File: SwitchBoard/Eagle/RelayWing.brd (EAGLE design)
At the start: 51.7 x 55.9 mm, 30 parts, among them K1 EE2-3TNUH, K2 EE2-3TNUH, K3 EE2-3TNUH, K4 EE2-3TNUH, K5 EE2-3TNUH, U1 ULN2003ANS, U2 ULN2003ANS, U3 MCP23017SS, U4 INA219AID

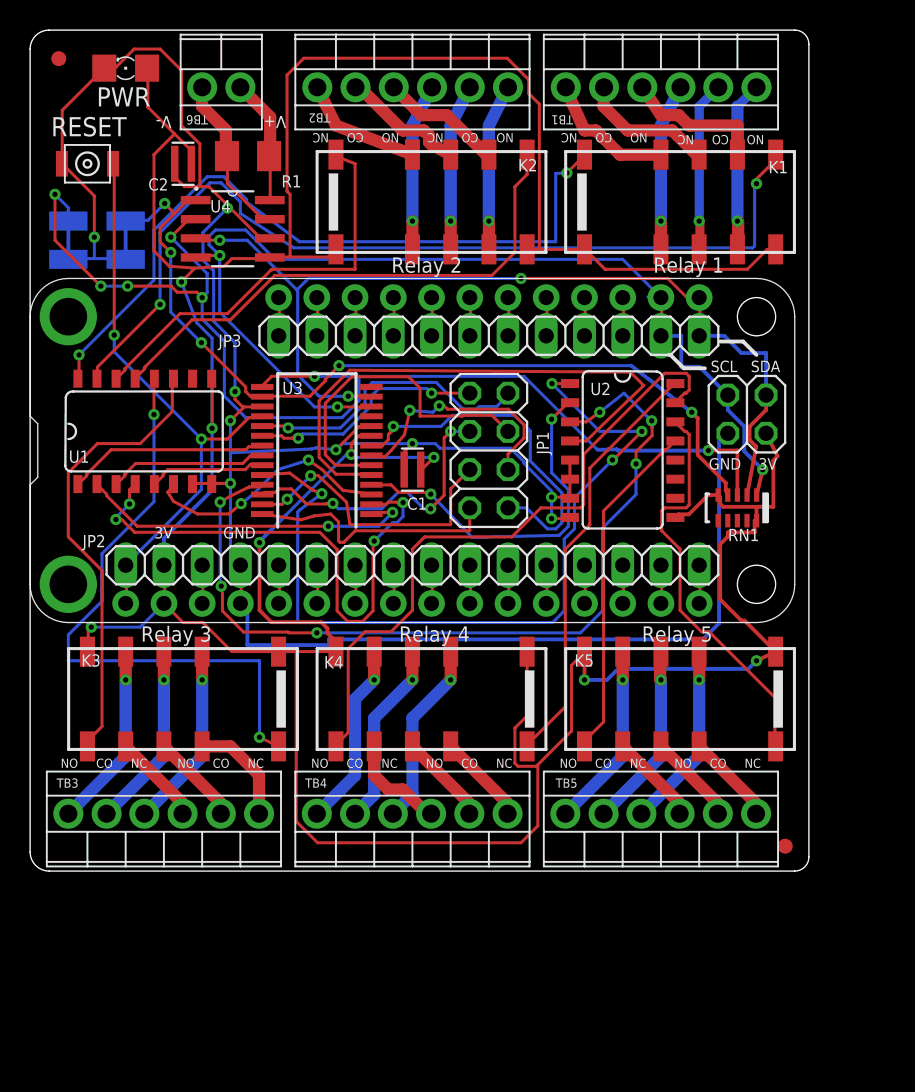
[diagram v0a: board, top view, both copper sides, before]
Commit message: Rev B (start)
First commit for Rev B. See updated Description.
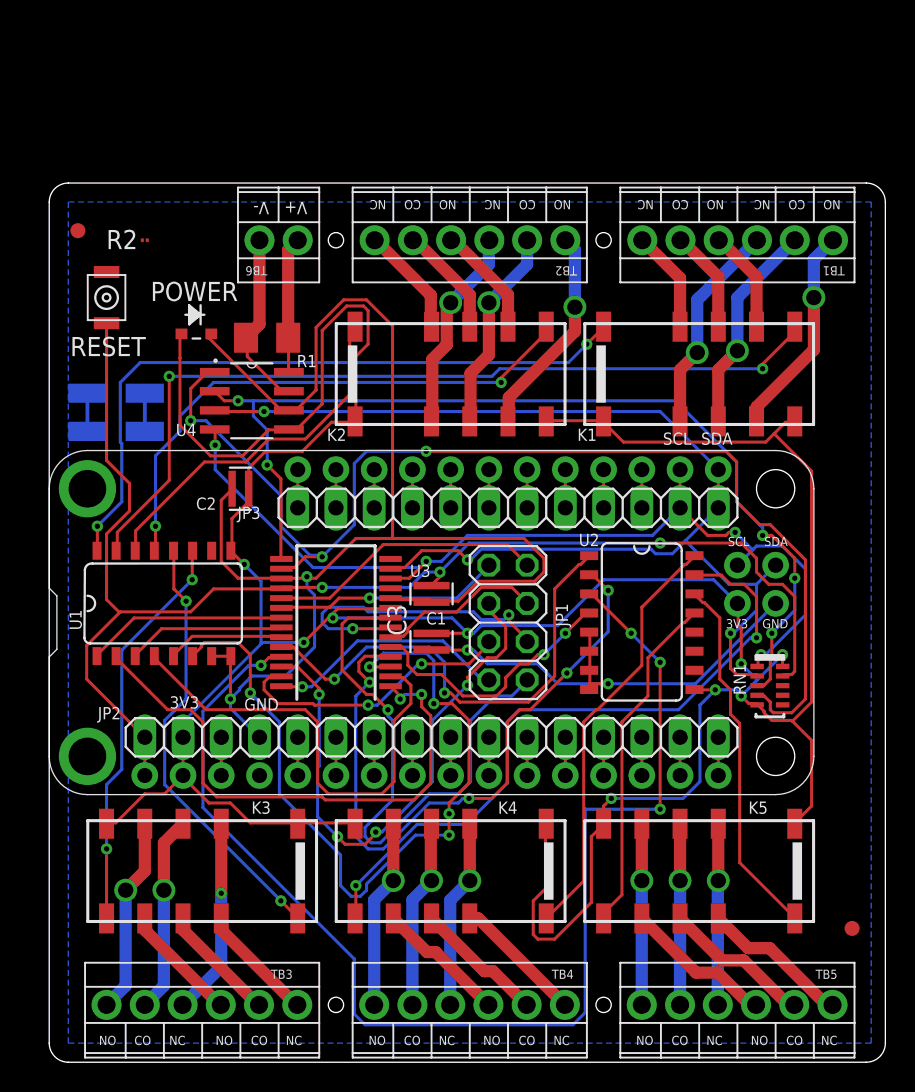
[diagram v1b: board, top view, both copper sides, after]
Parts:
- removed I2CHDR: (no value), pinhead:2X02
- removed PWR: (no value), led:1206
- added C3: MUR-1220-CAP, home:CAPC2012
- added JP4, JP5, JP6, JP7: (no value), adafruit:1X01-CLEANBIG
- added POWER: HSMQ-C191, DigiKey:LED3_HSMX-C120
- added R2: 330, home:R01005
- RN1: value CTS746X101 -> CTS746X101102JP
- moved C2 21.9 mm to (14.0, 39.4)
- moved TB5 13.7 mm to (47.0, 5.08)
- moved TB4 13.3 mm to (29.2, 5.08)
- moved TB3 13.0 mm to (11.4, 5.08)
- moved R1 12.1 mm to (15.7, 49.4)
- moved RN1 12.0 mm to (49.1, 26.3), turned to 270 degrees
- moved A0 11.5 mm to (3.81, 44.5)
- moved A1 11.5 mm to (7.62, 44.5)
- moved C1 11.5 mm to (26.7, 29.2), turned to 270 degrees
- moved JP2 11.5 mm to (26.7, 22.9)
- moved JP3 11.5 mm to (31.8, 38.1)
- moved K1 11.5 mm to (44.5, 47.0)
- moved K2 11.5 mm to (27.9, 47.0)
- moved MS1 11.5 mm to (1.27, 19.1)
- moved U1 11.5 mm to (8.89, 31.8)
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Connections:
- net N$16 renamed K1A-NO
- net N$17 renamed K2A-NO
- net N$2 renamed K4B-NO
- net N$24 renamed K1-SET
- net N$25 renamed K4B-NC
- net N$26 renamed K2A-CO
- net N$27 renamed K2A-NC
- net N$28 renamed K1A-NC
- net N$29 renamed K1B-NC
- net N$30 renamed K1A-CO
- net N$32 renamed K1B-CO
- net N$33 renamed K2B-CO
- net N$34 renamed K1-RESET
- net N$35 renamed K1B-NO
- net N$36 renamed K2-SET
- net N$37 renamed K2-RESET
- net N$38 renamed K3-SET
- net N$39 renamed K3-RESET
- net N$40 renamed K4A-CO
- net N$42 renamed K4A-N0
- net N$43 renamed K5A-CO
- net N$44 renamed K5A-NO
- net N$45 renamed K5B-NC
- net N$46 renamed K5B-CO
- net N$47 renamed K5B-NO
- net N$49 renamed K4B-CO
- net N$50 renamed K5A-NC
- net N$52 renamed K3A-NO
- net N$53 renamed K3A-NC
- net N$54 renamed K3A-CO
- net N$55 renamed K3B-NO
- net N$56 renamed K3B-NC
- net N$57 renamed K3B-CO
- net N$58 renamed K4-SET
- net N$59 renamed K4-RESET
- net N$60 renamed K5-SET
- net N$72 renamed K2B-NO
- net N$73 renamed K5-RESET
- net N$78 renamed K2B-NC
- net N$79 renamed K4A-NC
- removed net N$18: JP2.1, MS1.1, RESET.P$2, U3.18
- new net N$31: R2.2, RESET.P$1
- new net RESET/: C3.2, JP2.1, MS1.1, RESET.P$2, RN1.9, U3.18
- net 3V: now also JP4.1, POWER.2; no longer I2CHDR.3, PWR.A
- net GND: now also C3.1, JP5.1, POWER.1, R2.1; no longer I2CHDR.1, PWR.C, RESET.P$1
- net SCL: now also JP6.1; no longer I2CHDR.2
- net SDA: now also JP7.1; no longer I2CHDR.4
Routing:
- net RESET/: track 0.00 -> 90.0 mm, vias 0 -> 3
- net N$18: track 38.5 -> 0.00 mm, vias 2 -> 0
- net N$66: track 16.8 -> 51.9 mm, vias 2 -> 5
- net 3V: track 256.6 -> 224.6 mm, vias 8 -> 9
- net GND: track 158.2 -> 127.2 mm, vias 9 -> 4
- net N$70: track 57.7 -> 81.8 mm, vias 6 -> 4
- net N$68: track 54.3 -> 32.3 mm, vias 4 -> 2
- net N$69: track 24.1 -> 44.4 mm, vias 2 -> 4
- net N$71: track 36.9 -> 17.7 mm, vias 0 -> 2
- net A1: track 58.6 -> 76.5 mm, vias 5 -> 3
- net N$80: track 19.8 -> 36.5 mm, vias 3 -> 4
- net A0: track 80.2 -> 66.0 mm, vias 7 -> 5
- net N$77: track 23.6 -> 37.7 mm
- net N$63: track 22.7 -> 36.6 mm
- net SDA: track 64.6 -> 78.0 mm
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- added copper zone on layer 16, net GND
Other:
- board size 51.7 x 55.9 mm -> 55.5 x 58.4 mm
- board text added: "3V3"
- board text added: "Current Sensor: 2A @ 0-24V DC Only"
- board text added: "Relays: 2A @ +/-24V AC/DC"
- board text removed: "3V"
- board text removed: "Current Sensor: 2A @ 0-24V DC ONLY"
- board text removed: "I2C ADDR"
- board text removed: "Relay 1"
- board text removed: "Relay 2"
- board text removed: "Relay 3"
- board text removed: "Relay 4"
- board text removed: "Relay 5"
- board text removed: "Relay Switches: 2A @ +/- 24V AC/DC"
